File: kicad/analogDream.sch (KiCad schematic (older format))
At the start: 125 parts, among them P1 CONN_4X2, P10 CONN_7X2, P11 CONN_4X2, P12 CONN_4X2, P2 CONN_4X2, P3 CONN_7X2, P4 CONN_7X2, P5 CONN_4X2, P6 CONN_4X2, P7 CONN_4X2, P8 CONN_4X2, P9 CONN_7X2, U1 AD8221, U10 LT1026, U2 TL072, U3 AD8221, U4 TL072, U5 AD8221, U6 TL072, U7 AD8221, U8 TL072, U9 LT1026

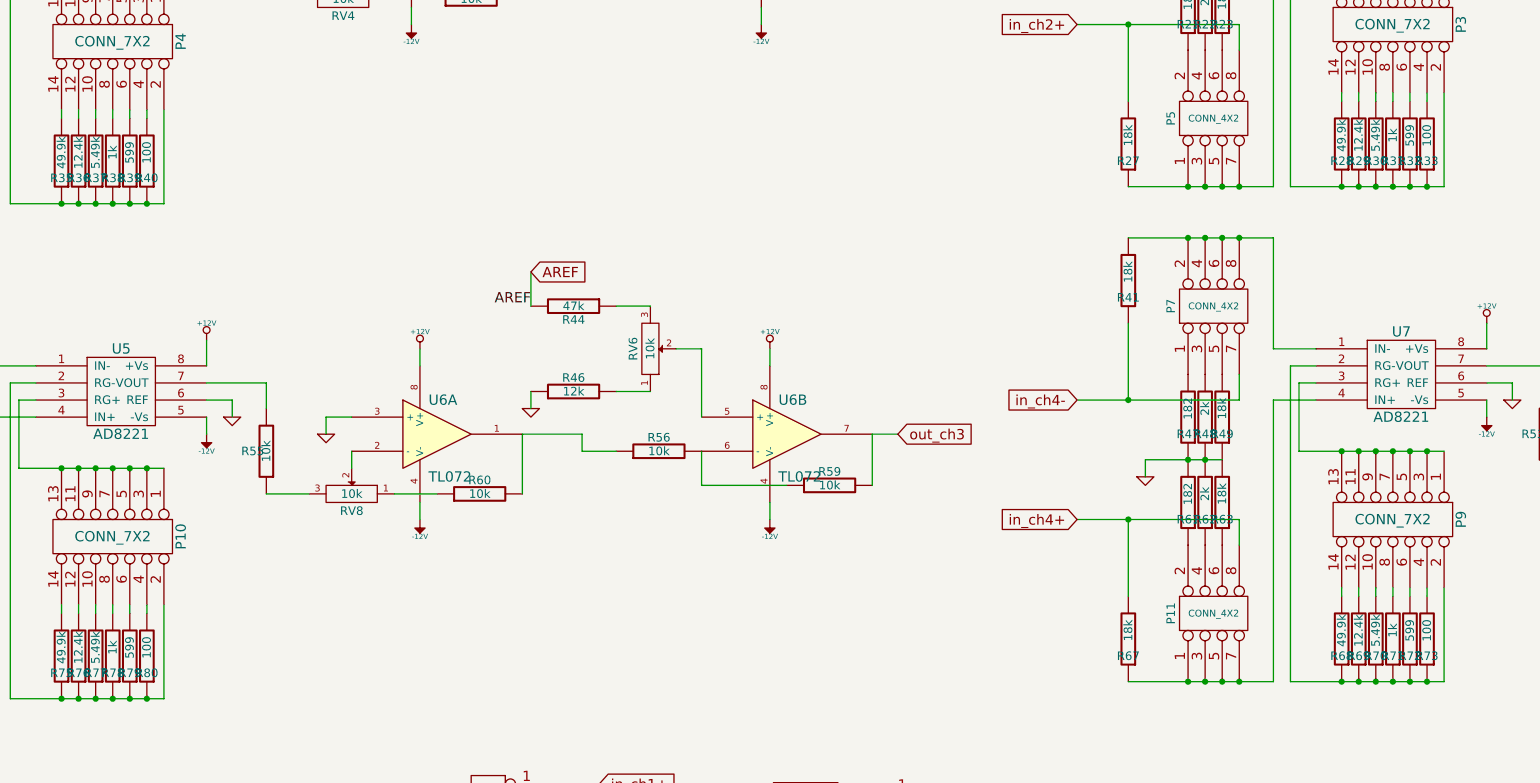
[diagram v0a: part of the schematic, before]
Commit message: Fixed Pot, worked on silk screen
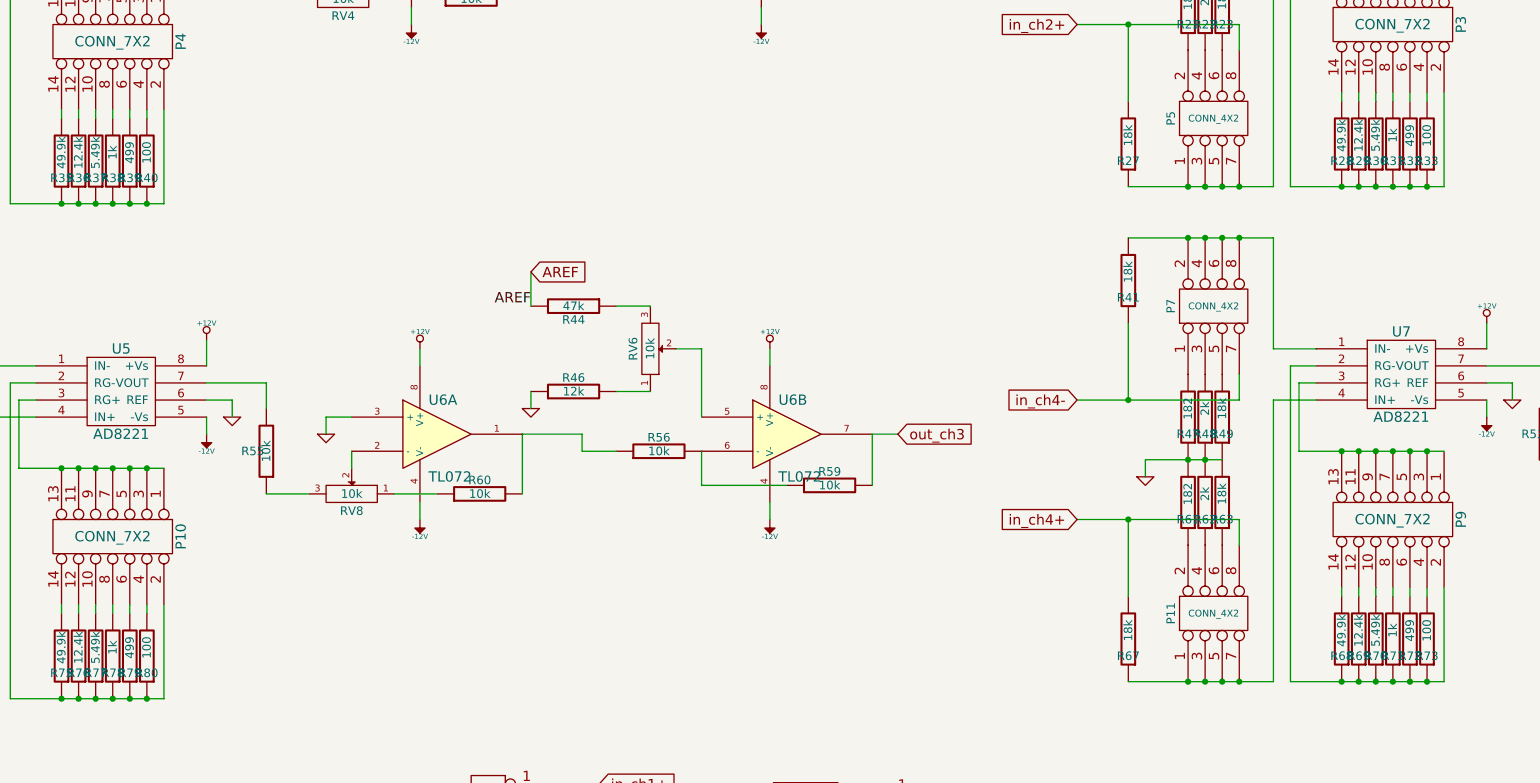
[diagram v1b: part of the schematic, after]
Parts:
- R32, R39, R72, R79: value 599 -> 499
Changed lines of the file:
@@
-EESchema Schematic File Version 2  date Sat 17 Dec 2011 09:17:39 PM MST
+EESchema Schematic File Version 2  date Fri 13 Jan 2012 09:39:40 PM MST
 LIBS:power
 LIBS:device
@@
 Sheet 1 1
 Title "Analog Dream Board"
-Date "18 dec 2011"
+Date "14 jan 2012"
 Rev ""
 Comp "Visgence Technologies"
@@
 P 10500 5850
 F 0 "R72" H 10500 5950 50  0000 C CNN
-F 1 "599" V 10500 5800 50  0000 C CNN
+F 1 "499" V 10500 5800 50  0000 C CNN
 	1    10500 5850
 	-1   0    0    1
@@
 P 10500 2950
 F 0 "R32" H 10500 3050 50  0000 C CNN
-F 1 "599" V 10500 2900 50  0000 C CNN
+F 1 "499" V 10500 2900 50  0000 C CNN
 	1    10500 2950
 	-1   0    0    1
@@
 P 3000 5950
 F 0 "R79" H 3000 6050 50  0000 C CNN
-F 1 "599" V 3000 5900 50  0000 C CNN
+F 1 "499" V 3000 5900 50  0000 C CNN
 	1    3000 5950
 	-1   0    0    1
@@
 P 3000 3050
 F 0 "R39" H 3000 3150 50  0000 C CNN
-F 1 "599" V 3000 3000 50  0000 C CNN
+F 1 "499" V 3000 3000 50  0000 C CNN
 	1    3000 3050
 	-1   0    0    1
